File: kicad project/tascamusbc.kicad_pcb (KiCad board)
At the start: 2 copper layers, 8.6 x 9.2 mm, 4 parts, among them J1 USB_B_Mini, J2 USB_C_Receptacle_USB2.0

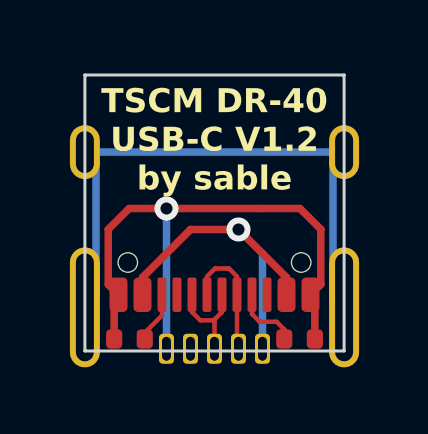
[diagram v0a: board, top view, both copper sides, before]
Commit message: updated schematic
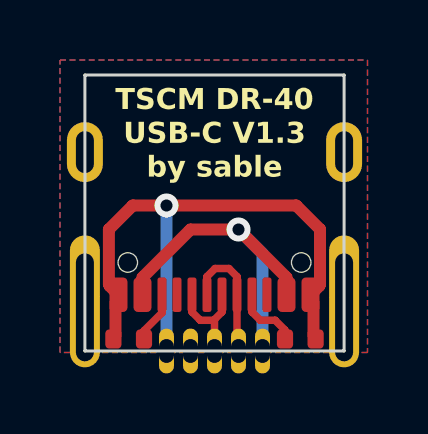
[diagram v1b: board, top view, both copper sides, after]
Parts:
- moved J1 0.07 mm to (64.4, 72.3)
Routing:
- net /SHIELD: track 19.6 -> 1.95 mm
- net /GND: track 20.1 -> 19.4 mm
- added copper zone on B.Cu, net /SHIELD
- added copper zone on F.Cu, net /SHIELD
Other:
- board text added: "TSCM DR-40 USB-C V1.3 by sable"
- board text added: "who needs clearences, lol?"
- board text removed: "TSCM DR-40 USB-C V1.2 by sable"
- board text removed: "hopefully i'm only seen once"
